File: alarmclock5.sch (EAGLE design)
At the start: 39 parts, among them X1 MKDSN1,5/2-5,08, X2 MKDSN1,5/2-5,08, X3 MKDSN1,5/2-5,08, X4 MKDSN1,5/2-5,08

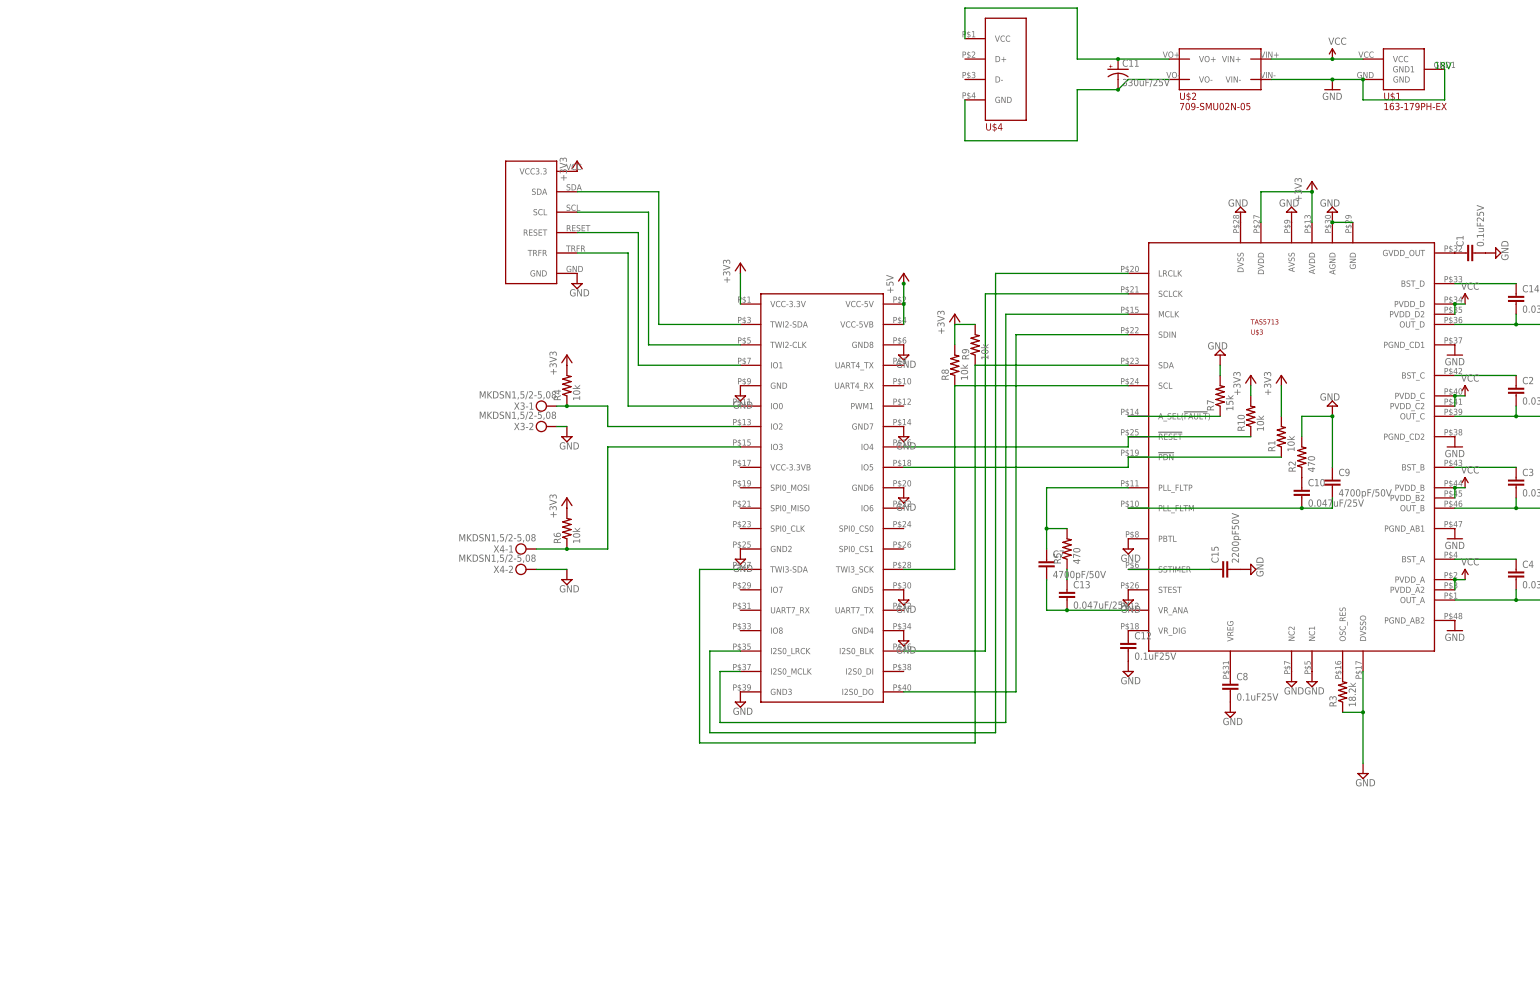
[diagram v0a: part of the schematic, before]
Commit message: new schema
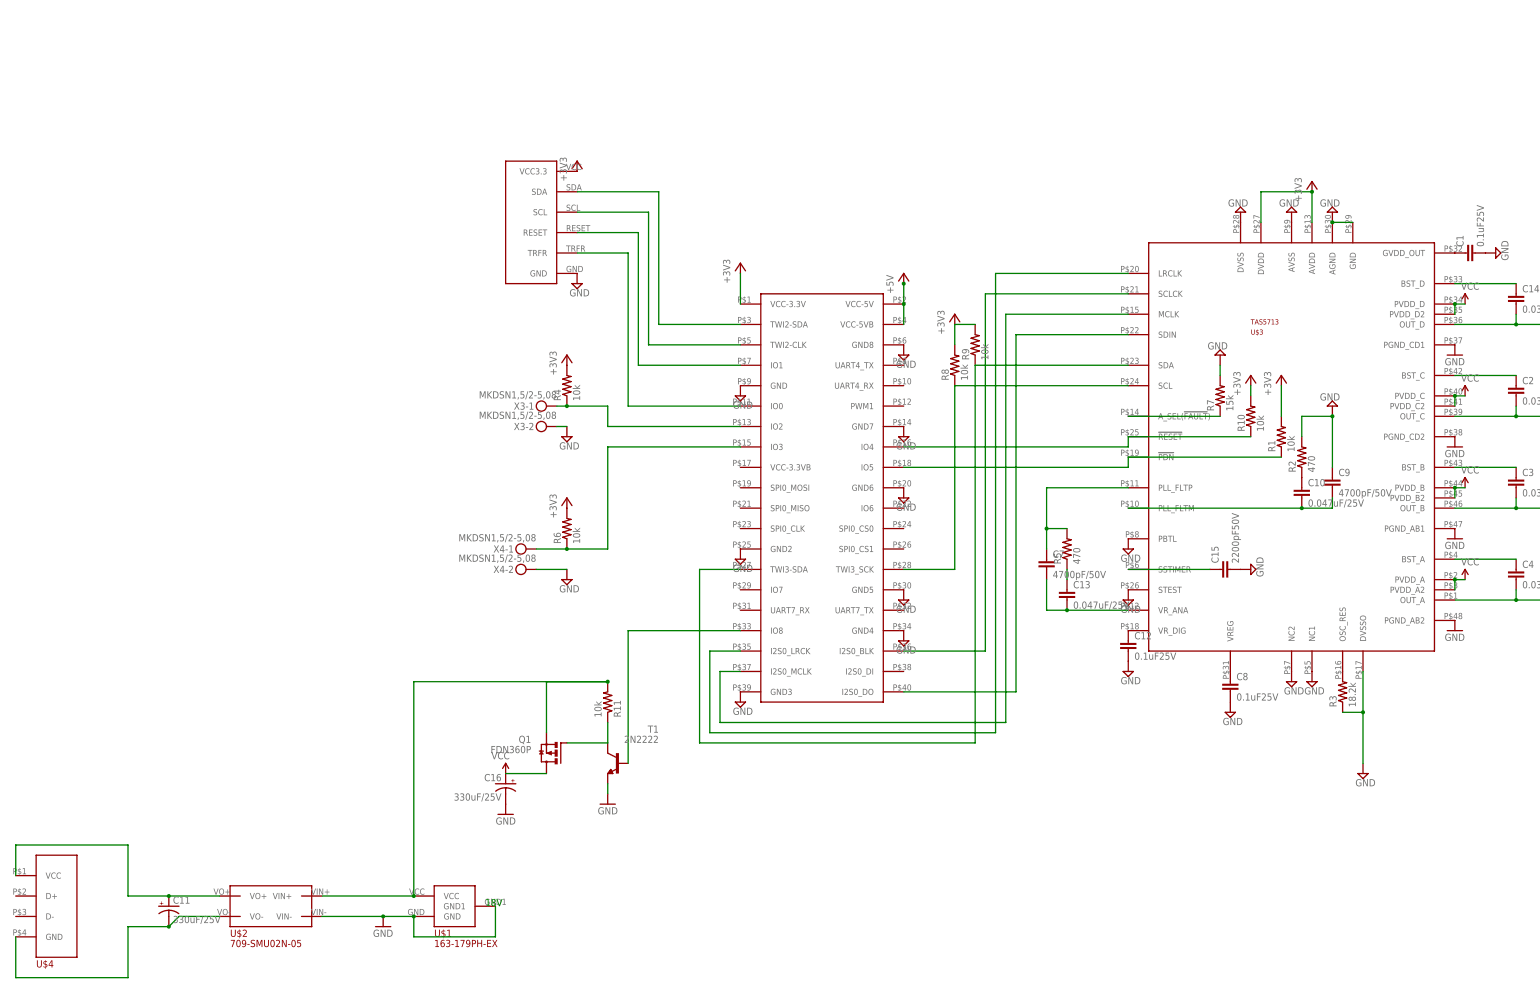
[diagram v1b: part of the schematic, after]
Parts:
- added C16: 330uF/25V, SparkFun-Passives:CAP_POLPTH2
- added Q1: FDN360P, transistor-power:FDN360P
- added R11: 10k, SparkFun-Passives:RESISTOR0603-RES
- added T1: 2N2222, transistor:2N2222
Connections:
- new net N$40: T1.B, U$5.IO8
- new net N$41: Q1.G, R11.1, T1.C
- new net N$43: Q1.S, R11.2, U$1.VCC, U$2.VIN+
- net GND: now also C16.-, T1.E
- net VCC: now also C16.+, Q1.D; no longer U$1.VCC, U$2.VIN+
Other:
- moved on the sheet: C11, U$1, U$2, U$4
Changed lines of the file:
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@@
 <part name="U$1" library="mouser" deviceset="163-179PH-EX" device=""/>
 <part name="U$2" library="mouser" deviceset="709-SMU02N-05" device=""/>
-<part name="SUPPLY1" library="SparkFun-Aesthetics" deviceset="VCC" device=""/>
 <part name="GND1" library="SparkFun-Aesthetics" deviceset="GND" device=""/>
 <part name="U$4" library="mouser" deviceset="USB_TYPEA_CONNECTOR" device=""/>
@@
 <part name="C15" library="SparkFun-Capacitors" deviceset="CAP" device="0603-CAP" value="2200pF50V"/>
 <part name="SUPPLY30" library="supply2" deviceset="GND" device=""/>
+<part name="T1" library="transistor" deviceset="2N2222" device=""/>
+<part name="GND2" library="SparkFun-Aesthetics" deviceset="GND" device=""/>
+<part name="R11" library="SparkFun-Passives" deviceset="RESISTOR" device="0603-RES" value="10k"/>
+<part name="Q1" library="transistor-power" deviceset="FDN360P" device=""/>
+<part name="GND3" library="SparkFun-Aesthetics" deviceset="GND" device=""/>
+<part name="SUPPLY31" library="SparkFun-Aesthetics" deviceset="VCC" device=""/>
+<part name="C16" library="SparkFun-Passives" deviceset="CAP_POL" device="PTH2" value="330uF/25V"/>
 </parts>
 <sheets>
 <sheet>
 <plain>
-<text x="152.4" y="76.2" size="1.778" layer="91">18V</text>
+<text x="-83.82" y="-132.08" size="1.778" layer="91">18V</text>
 </plain>
 <instances>
-<instance part="U$1" gate="G$1" x="139.7" y="76.2"/>
-<instance part="U$2" gate="G$1" x="96.52" y="73.66"/>
-<instance part="SUPPLY1" gate="G$1" x="127" y="78.74"/>
-<instance part="GND1" gate="1" x="127" y="71.12"/>
-<instance part="U$4" gate="G$1" x="45.72" y="76.2"/>
+<instance part="U$1" gate="G$1" x="-96.52" y="-132.08"/>
+<instance part="U$2" gate="G$1" x="-139.7" y="-134.62"/>
+<instance part="GND1" gate="1" x="-109.22" y="-137.16"/>
+<instance part="U$4" gate="G$1" x="-190.5" y="-132.08"/>
 <instance part="U$3" gate="G$1" x="116.84" y="-17.78"/>
 <instance part="GND4" gate="1" x="157.48" y="-63.5"/>
@@
 <instance part="R3" gate="G$1" x="129.54" y="-78.74" rot="R90"/>
 <instance part="R1" gate="G$1" x="114.3" y="-15.24" rot="R90"/>
-<instance part="C11" gate="G$1" x="73.66" y="76.2"/>
+<instance part="C11" gate="G$1" x="-162.56" y="-132.08"/>
 <instance part="SUPPLY6" gate="GND" x="127" y="-7.62" rot="R180"/>
 <instance part="+3V1" gate="G$1" x="-20.32" y="27.94"/>
@@
 <instance part="C15" gate="G$1" x="101.6" y="-48.26" rot="R90"/>
 <instance part="SUPPLY30" gate="GND" x="106.68" y="-48.26" rot="R90"/>
+<instance part="T1" gate="G$1" x="-50.8" y="-96.52" rot="MR0"/>
+<instance part="GND2" gate="1" x="-53.34" y="-106.68" rot="MR0"/>
+<instance part="R11" gate="G$1" x="-53.34" y="-81.28" rot="MR90"/>
+<instance part="Q1" gate="G$1" x="-66.04" y="-93.98" rot="MR0"/>
+<instance part="GND3" gate="1" x="-78.74" y="-109.22" rot="MR0"/>
+<instance part="SUPPLY31" gate="G$1" x="-78.74" y="-99.06" rot="MR0"/>
+<instance part="C16" gate="G$1" x="-78.74" y="-101.6" rot="MR0"/>
 </instances>
 <busses>
@@
 <segment>
 <pinref part="U$2" gate="G$1" pin="VO+"/>
-<wire x1="63.5" y1="78.74" x2="73.66" y2="78.74" width="0.1524" layer="91"/>
+<wire x1="-172.72" y1="-129.54" x2="-162.56" y2="-129.54" width="0.1524" layer="91"/>
 <pinref part="U$4" gate="G$1" pin="VCC"/>
-<wire x1="73.66" y1="78.74" x2="86.36" y2="78.74" width="0.1524" layer="91"/>
-<wire x1="35.56" y1="83.82" x2="35.56" y2="91.44" width="0.1524" layer="91"/>
-<wire x1="35.56" y1="91.44" x2="63.5" y2="91.44" width="0.1524" layer="91"/>
-<wire x1="63.5" y1="91.44" x2="63.5" y2="78.74" width="0.1524" layer="91"/>
+<wire x1="-162.56" y1="-129.54" x2="-149.86" y2="-129.54" width="0.1524" layer="91"/>
+<wire x1="-200.66" y1="-124.46" x2="-200.66" y2="-116.84" width="0.1524" layer="91"/>
+<wire x1="-200.66" y1="-116.84" x2="-172.72" y2="-116.84" width="0.1524" layer="91"/>
+<wire x1="-172.72" y1="-116.84" x2="-172.72" y2="-129.54" width="0.1524" layer="91"/>
 <pinref part="C11" gate="G$1" pin="+"/>
-<junction x="73.66" y="78.74"/>
+<junction x="-162.56" y="-129.54"/>
 </segment>
 </net>
 <net name="VCC" class="1">
-<segment>
-<pinref part="U$2" gate="G$1" pin="VIN+"/>
-<pinref part="U$1" gate="G$1" pin="VCC"/>
-<wire x1="111.76" y1="78.74" x2="127" y2="78.74" width="0.1524" layer="91"/>
-<pinref part="SUPPLY1" gate="G$1" pin="VCC"/>
-<wire x1="127" y1="78.74" x2="134.62" y2="78.74" width="0.1524" layer="91"/>
-<junction x="127" y="78.74"/>
-</segment>
 <segment>
 <pinref part="SUPPLY5" gate="G$1" pin="VCC"/>
@@
 <junction x="157.48" y="-50.8"/>
 </segment>
+<segment>
+<pinref part="SUPPLY31" gate="G$1" pin="VCC"/>
+<pinref part="C16" gate="G$1" pin="+"/>
+<pinref part="Q1" gate="G$1" pin="D"/>
+<wire x1="-68.58" y1="-99.06" x2="-78.74" y2="-99.06" width="0.1524" layer="91"/>
+</segment>
 </net>
 <net name="GND" class="1">
@@
 <pinref part="U$1" gate="G$1" pin="GND"/>
 <pinref part="U$2" gate="G$1" pin="VIN-"/>
-<wire x1="134.62" y1="73.66" x2="127" y2="73.66" width="0.1524" layer="91"/>
+<wire x1="-101.6" y1="-134.62" x2="-109.22" y2="-134.62" width="0.1524" layer="91"/>
 <pinref part="GND1" gate="1" pin="GND"/>
-<wire x1="127" y1="73.66" x2="111.76" y2="73.66" width="0.1524" layer="91"/>
-<junction x="127" y="73.66"/>
-<wire x1="134.62" y1="73.66" x2="134.62" y2="68.58" width="0.1524" layer="91"/>
-<wire x1="134.62" y1="68.58" x2="154.94" y2="68.58" width="0.1524" layer="91"/>
+<wire x1="-109.22" y1="-134.62" x2="-124.46" y2="-134.62" width="0.1524" layer="91"/>
+<junction x="-109.22" y="-134.62"/>
+<wire x1="-101.6" y1="-134.62" x2="-101.6" y2="-139.7" width="0.1524" layer="91"/>
+<wire x1="-101.6" y1="-139.7" x2="-81.28" y2="-139.7" width="0.1524" layer="91"/>
 <pinref part="U$1" gate="G$1" pin="GND1"/>
-<wire x1="154.94" y1="68.58" x2="154.94" y2="76.2" width="0.1524" layer="91"/>
-<junction x="134.62" y="73.66"/>
+<wire x1="-81.28" y1="-139.7" x2="-81.28" y2="-132.08" width="0.1524" layer="91"/>
+<junction x="-101.6" y="-134.62"/>
 </segment>
 <segment>
@@
 <pinref part="C15" gate="G$1" pin="2"/>
 <pinref part="SUPPLY30" gate="GND" pin="GND"/>
+</segment>
+<segment>
+<pinref part="T1" gate="G$1" pin="E"/>
+<pinref part="GND2" gate="1" pin="GND"/>
+<wire x1="-53.34" y1="-104.14" x2="-53.34" y2="-101.6" width="0.1524" layer="91"/>
+</segment>
+<segment>
+<pinref part="C16" gate="G$1" pin="-"/>
+<pinref part="GND3" gate="1" pin="GND"/>
 </segment>
 </net>
@@
 <segment>
 <pinref part="U$2" gate="G$1" pin="VO-"/>
-<wire x1="86.36" y1="73.66" x2="76.2" y2="73.66" width="0.1524" layer="91"/>
-<wire x1="76.2" y1="73.66" x2="73.66" y2="71.12" width="0.1524" layer="91"/>
-<wire x1="73.66" y1="71.12" x2="63.5" y2="71.12" width="0.1524" layer="91"/>
+<wire x1="-149.86" y1="-134.62" x2="-160.02" y2="-134.62" width="0.1524" layer="91"/>
+<wire x1="-160.02" y1="-134.62" x2="-162.56" y2="-137.16" width="0.1524" layer="91"/>
+<wire x1="-162.56" y1="-137.16" x2="-172.72" y2="-137.16" width="0.1524" layer="91"/>
 <pinref part="U$4" gate="G$1" pin="GND"/>
-<wire x1="35.56" y1="68.58" x2="35.56" y2="58.42" width="0.1524" layer="91"/>
-<wire x1="35.56" y1="58.42" x2="63.5" y2="58.42" width="0.1524" layer="91"/>
-<wire x1="63.5" y1="58.42" x2="63.5" y2="71.12" width="0.1524" layer="91"/>
+<wire x1="-200.66" y1="-139.7" x2="-200.66" y2="-149.86" width="0.1524" layer="91"/>
+<wire x1="-200.66" y1="-149.86" x2="-172.72" y2="-149.86" width="0.1524" layer="91"/>
+<wire x1="-172.72" y1="-149.86" x2="-172.72" y2="-137.16" width="0.1524" layer="91"/>
 <pinref part="C11" gate="G$1" pin="-"/>
-<junction x="73.66" y="71.12"/>
+<junction x="-162.56" y="-137.16"/>
 </segment>
 </net>
@@
 </segment>
 </net>
+<net name="N$40" class="0">
+<segment>
+<pinref part="U$5" gate="G$1" pin="IO8"/>
+<wire x1="-20.32" y1="-63.5" x2="-48.26" y2="-63.5" width="0.1524" layer="91"/>
+<pinref part="T1" gate="G$1" pin="B"/>
+<wire x1="-48.26" y1="-63.5" x2="-48.26" y2="-96.52" width="0.1524" layer="91"/>
+</segment>
+</net>
+<net name="N$41" class="0">
+<segment>
+<pinref part="T1" gate="G$1" pin="C"/>
+<pinref part="R11" gate="G$1" pin="1"/>
+<wire x1="-53.34" y1="-86.36" x2="-53.34" y2="-91.44" width="0.1524" layer="91"/>
+<pinref part="Q1" gate="G$1" pin="G"/>
+<wire x1="-63.5" y1="-91.44" x2="-53.34" y2="-91.44" width="0.1524" layer="91"/>
+</segment>
+</net>
+<net name="N$43" class="0">
+<segment>
+<pinref part="U$1" gate="G$1" pin="VCC"/>
+<pinref part="U$2" gate="G$1" pin="VIN+"/>
+<wire x1="-101.6" y1="-129.54" x2="-124.46" y2="-129.54" width="0.1524" layer="91"/>
+<wire x1="-101.6" y1="-129.54" x2="-101.6" y2="-76.2" width="0.1524" layer="91"/>
+<pinref part="Q1" gate="G$1" pin="S"/>
+<wire x1="-68.58" y1="-88.9" x2="-68.58" y2="-76.2" width="0.1524" layer="91"/>
+<pinref part="R11" gate="G$1" pin="2"/>
+<wire x1="-68.58" y1="-76.2" x2="-53.34" y2="-76.2" width="0.1524" layer="91"/>
+<wire x1="-101.6" y1="-76.2" x2="-53.34" y2="-76.2" width="0.1524" layer="91"/>
+<junction x="-53.34" y="-76.2"/>
+<junction x="-101.6" y="-129.54"/>
+</segment>
+</net>
